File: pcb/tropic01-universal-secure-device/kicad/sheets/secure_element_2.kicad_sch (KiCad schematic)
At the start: 0 parts

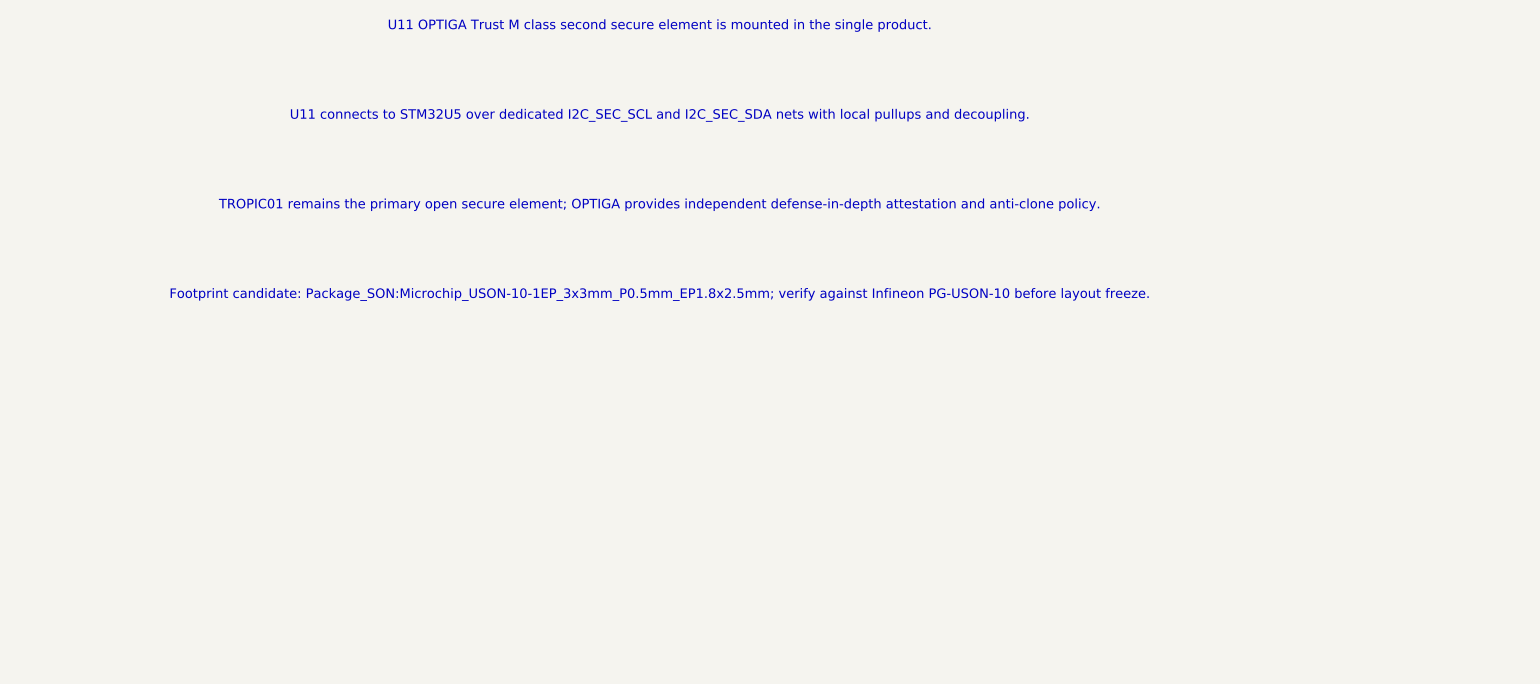
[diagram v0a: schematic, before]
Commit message: feat: materialize tropic01 schematic bindings
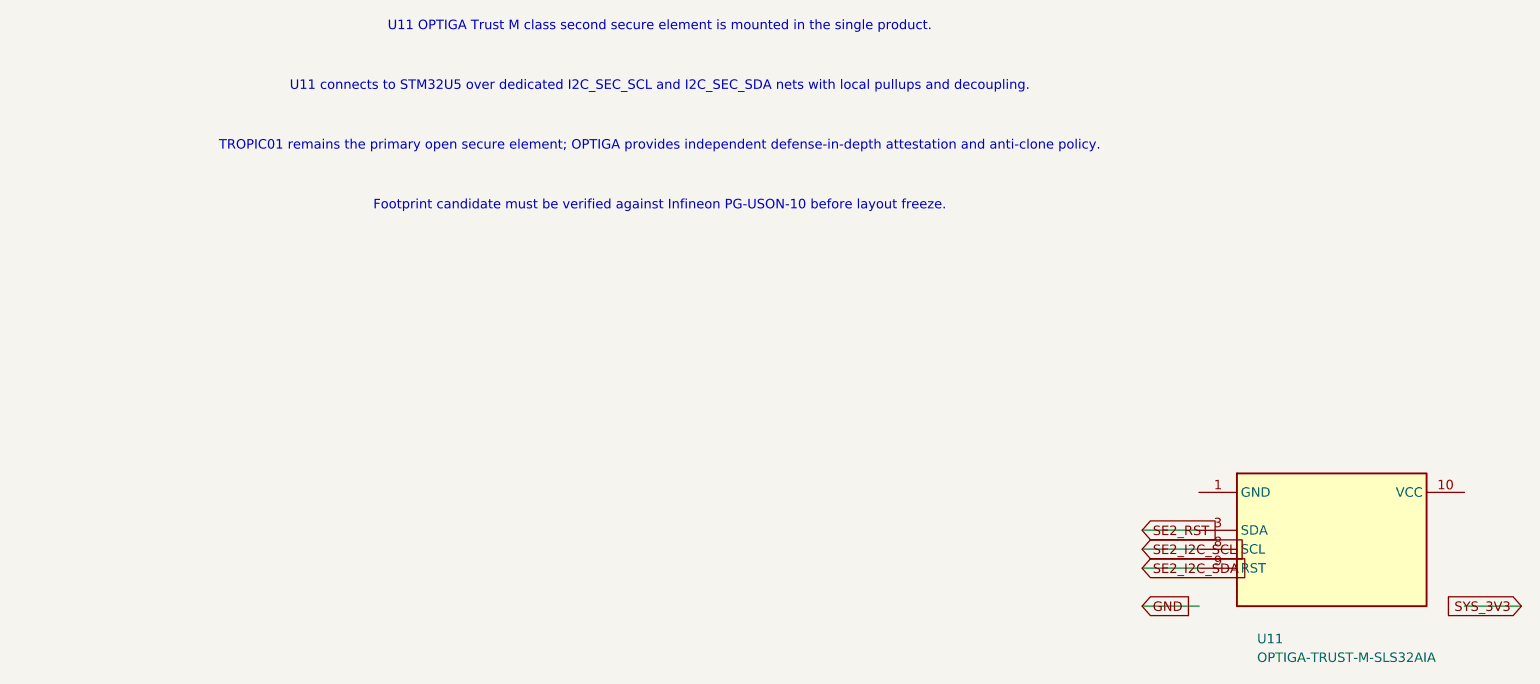
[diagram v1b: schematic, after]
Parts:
- added U11: OPTIGA-TRUST-M-SLS32AIA, Package_SON:Microchip_USON-10-1EP_3x3mm_P0.5mm_EP1.8x2.5mm, symbol TROPIC_SQUARE:OPTIGA_TRUST_M_USON10
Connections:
- new net SE2_I2C_SCL: U11.8 (SCL)
- new net SE2_I2C_SDA: U11.9 (RST)
- new net SE2_RST: U11.3 (SDA)
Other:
- note added: "Footprint candidate must be verified against Infineon PG-USON-10 before layout freeze."
- note removed: "Footprint candidate: Package_SON:Microchip_USON-10-1EP_3x3mm_P0.5mm_EP1.8x2.5mm; verify against Infineon PG-USON-10 before layout freeze."
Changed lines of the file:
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@@
 	(text "U11 OPTIGA Trust M class second secure element is mounted in the single product."
 		(exclude_from_sim no)
-		(at 20 20 0)
-		(effects
-			(font
-				(size 1.27 1.27)
+		(at 20.00 20.00 0)
+		(effects (font (size 1.27 1.27)))
+	)
+	(text "U11 connects to STM32U5 over dedicated I2C_SEC_SCL and I2C_SEC_SDA nets with local pullups and decoupling."
+		(exclude_from_sim no)
+		(at 20.00 28.00 0)
+		(effects (font (size 1.27 1.27)))
+	)
+	(text "TROPIC01 remains the primary open secure element; OPTIGA provides independent defense-in-depth attestation and anti-clone policy."
+		(exclude_from_sim no)
+		(at 20.00 36.00 0)
+		(effects (font (size 1.27 1.27)))
+	)
+	(text "Footprint candidate must be verified against Infineon PG-USON-10 before layout freeze."
+		(exclude_from_sim no)
+		(at 20.00 44.00 0)
+		(effects (font (size 1.27 1.27)))
+	)
+	(symbol
+		(lib_id "TROPIC_SQUARE:OPTIGA_TRUST_M_USON10")
+		(at 110.00 90.00 0)
+		(unit 1)
+		(exclude_from_sim no)
+		(in_bom yes)
+		(on_board yes)
+		(dnp no)
+		(property "Reference" "U11"
+			(at 100.00 102.00 0)
+			(effects (font (size 1.27 1.27)) (justify left))
+		)
+		(property "Value" "OPTIGA-TRUST-M-SLS32AIA"
+			(at 100.00 104.50 0)
+			(effects (font (size 1.27 1.27)) (justify left))
+		)
+		(property "Footprint" "Package_SON:Microchip_USON-10-1EP_3x3mm_P0.5mm_EP1.8x2.5mm"
+			(at 110.00 90.00 0)
+			(effects (font (size 1.27 1.27)) (hide yes))
+		)
+		(property "Datasheet" "https://www.infineon.com/assets/row/public/documents/30/49/infineon-optiga-trust-m-sls32aia-datasheet-en.pdf"
+			(at 110.00 90.00 0)
+			(effects (font (size 1.27 1.27)) (hide yes))
+		)
+		(property "Description" "OPTIGA Trust M class second secure element, PG-USON-10 candidate footprint"
+			(at 110.00 90.00 0)
+			(effects (font (size 1.27 1.27)) (hide yes))
+		)
+		(instances
+			(project "tropic01-universal-secure-device"
+				(path "/11111111-1111-4111-8111-111111111111/88888888-8888-4888-8888-777777777777"
+					(reference "U11")
+					(unit 1)
+				)
 			)
 		)
 	)
-	(text "U11 connects to STM32U5 over dedicated I2C_SEC_SCL and I2C_SEC_SDA nets with local pullups and decoupling."
-		(exclude_from_sim no)
-		(at 20 32 0)
-		(effects
-			(font
-				(size 1.27 1.27)
-			)
+	(wire
+		(pts
+			(xy 92.22 97.62) (xy 84.60 97.62)
 		)
+		(stroke (width 0) (type default))
 	)
-	(text "TROPIC01 remains the primary open secure element; OPTIGA provides independent defense-in-depth attestation and anti-clone policy."
-		(exclude_from_sim no)
-		(at 20 44 0)
-		(effects
-			(font
-				(size 1.27 1.27)
-			)
+	(global_label "GND"
+		(shape input)
+		(at 84.60 97.62 0)
+		(fields_autoplaced)
+		(effects (font (size 1.27 1.27)))
+	)
+	(wire
+		(pts
+			(xy 127.78 97.62) (xy 135.40 97.62)
 		)
+		(stroke (width 0) (type default))
 	)
-	(text "Footprint candidate: Package_SON:Microchip_USON-10-1EP_3x3mm_P0.5mm_EP1.8x2.5mm; verify against Infineon PG-USON-10 before layout freeze."
-		(exclude_from_sim no)
-		(at 20 56 0)
-		(effects
-			(font
-				(size 1.27 1.27)
-			)
+	(global_label "SYS_3V3"
+		(shape input)
+		(at 135.40 97.62 180)
+		(fields_autoplaced)
+		(effects (font (size 1.27 1.27)))
+	)
+	(wire
+		(pts
+			(xy 92.22 92.54) (xy 84.60 92.54)
 		)
+		(stroke (width 0) (type default))
+	)
+	(global_label "SE2_I2C_SDA"
+		(shape input)
+		(at 84.60 92.54 0)
+		(fields_autoplaced)
+		(effects (font (size 1.27 1.27)))
+	)
+	(wire
+		(pts
+			(xy 92.22 90.00) (xy 84.60 90.00)
+		)
+		(stroke (width 0) (type default))
+	)
+	(global_label "SE2_I2C_SCL"
+		(shape input)
+		(at 84.60 90.00 0)
+		(fields_autoplaced)
+		(effects (font (size 1.27 1.27)))
+	)
+	(wire
+		(pts
+			(xy 92.22 87.46) (xy 84.60 87.46)
+		)
+		(stroke (width 0) (type default))
+	)
+	(global_label "SE2_RST"
+		(shape input)
+		(at 84.60 87.46 0)
+		(fields_autoplaced)
+		(effects (font (size 1.27 1.27)))
 	)
 	(sheet_instances

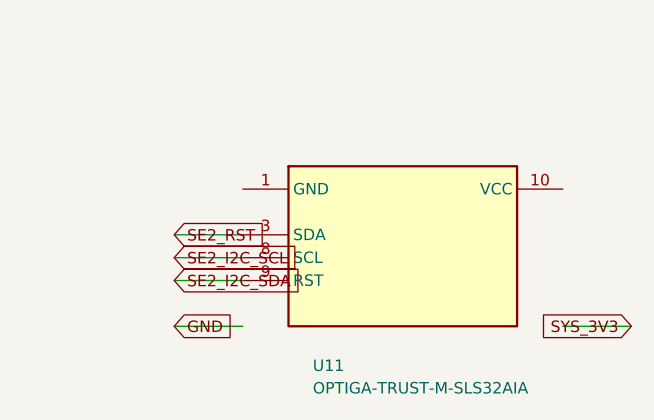
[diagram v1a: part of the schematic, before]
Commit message: feat: bind tropic01 pcb nets
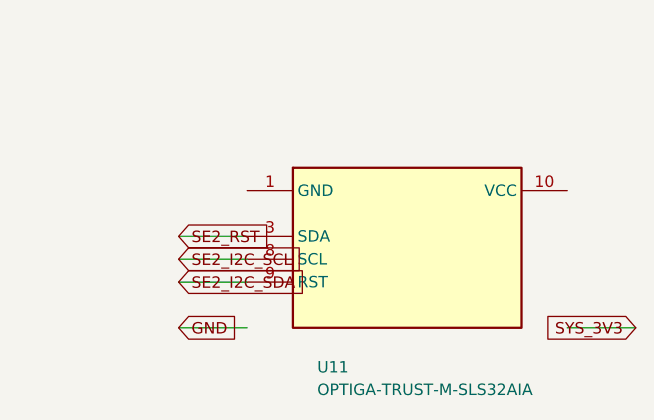
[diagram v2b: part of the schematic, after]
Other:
- moved on the sheet: U11
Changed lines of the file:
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@@
 	(symbol
 		(lib_id "TROPIC_SQUARE:OPTIGA_TRUST_M_USON10")
-		(at 110.00 90.00 0)
+		(at 110.49 90.17 0)
 		(unit 1)
 		(exclude_from_sim no)
@@
 		(dnp no)
 		(property "Reference" "U11"
-			(at 100.00 102.00 0)
+			(at 100.49 102.17 0)
 			(effects (font (size 1.27 1.27)) (justify left))
 		)
 		(property "Value" "OPTIGA-TRUST-M-SLS32AIA"
-			(at 100.00 104.50 0)
+			(at 100.49 104.67 0)
 			(effects (font (size 1.27 1.27)) (justify left))
 		)
 		(property "Footprint" "Package_SON:Microchip_USON-10-1EP_3x3mm_P0.5mm_EP1.8x2.5mm"
-			(at 110.00 90.00 0)
+			(at 110.49 90.17 0)
 			(effects (font (size 1.27 1.27)) (hide yes))
 		)
 		(property "Datasheet" "https://www.infineon.com/assets/row/public/documents/30/49/infineon-optiga-trust-m-sls32aia-datasheet-en.pdf"
-			(at 110.00 90.00 0)
+			(at 110.49 90.17 0)
 			(effects (font (size 1.27 1.27)) (hide yes))
 		)
 		(property "Description" "OPTIGA Trust M class second secure element, PG-USON-10 candidate footprint"
-			(at 110.00 90.00 0)
+			(at 110.49 90.17 0)
 			(effects (font (size 1.27 1.27)) (hide yes))
 		)
@@
 	(wire
 		(pts
-			(xy 92.22 97.62) (xy 84.60 97.62)
+			(xy 92.71 97.79) (xy 85.09 97.79)
 		)
 		(stroke (width 0) (type default))
@@
 	(global_label "GND"
 		(shape input)
-		(at 84.60 97.62 0)
+		(at 85.09 97.79 0)
 		(fields_autoplaced)
 		(effects (font (size 1.27 1.27)))
@@
 	(wire
 		(pts
-			(xy 127.78 97.62) (xy 135.40 97.62)
+			(xy 128.27 97.79) (xy 135.89 97.79)
 		)
 		(stroke (width 0) (type default))
@@
 	(global_label "SYS_3V3"
 		(shape input)
-		(at 135.40 97.62 180)
+		(at 135.89 97.79 180)
 		(fields_autoplaced)
 		(effects (font (size 1.27 1.27)))
@@
 	(wire
 		(pts
-			(xy 92.22 92.54) (xy 84.60 92.54)
+			(xy 92.71 92.71) (xy 85.09 92.71)
 		)
 		(stroke (width 0) (type default))
@@
 	(global_label "SE2_I2C_SDA"
 		(shape input)
-		(at 84.60 92.54 0)
+		(at 85.09 92.71 0)
 		(fields_autoplaced)
 		(effects (font (size 1.27 1.27)))
@@
 	(wire
 		(pts
-			(xy 92.22 90.00) (xy 84.60 90.00)
+			(xy 92.71 90.17) (xy 85.09 90.17)
 		)
 		(stroke (width 0) (type default))
@@
 	(global_label "SE2_I2C_SCL"
 		(shape input)
-		(at 84.60 90.00 0)
+		(at 85.09 90.17 0)
 		(fields_autoplaced)
 		(effects (font (size 1.27 1.27)))
@@
 	(wire
 		(pts
-			(xy 92.22 87.46) (xy 84.60 87.46)
+			(xy 92.71 87.63) (xy 85.09 87.63)
 		)
 		(stroke (width 0) (type default))
@@
 	(global_label "SE2_RST"
 		(shape input)
-		(at 84.60 87.46 0)
+		(at 85.09 87.63 0)
 		(fields_autoplaced)
 		(effects (font (size 1.27 1.27)))
